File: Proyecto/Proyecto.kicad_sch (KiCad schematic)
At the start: 48 parts, among them IC1 MC9S08MP16xLC, J1 Bomba1, J10 DHT11, J11 Bomba2, J12 Aux1, J13 LCD, J14 Aux2, J15 Expansion, J16 NIVEL BAJO, J17 NIVEL ALTO, J18 LDR, J2 Rele1, J3 Luces, J4 Rele2, J5 TDS, J6 Rele3, J7 Rele4, J8 ENTRADA, J9 PH, K1 FINDER-36.11, K2 FINDER-36.11, K3 FINDER-36.11, K4 FINDER-36.11, Q1 IRF3205, Q2 IRF3205, U1 ULN2803A, U2 MIC4427, U3 AP63205WU, U4 PC817, U5 PC817, U6 LM358, U7 LM358

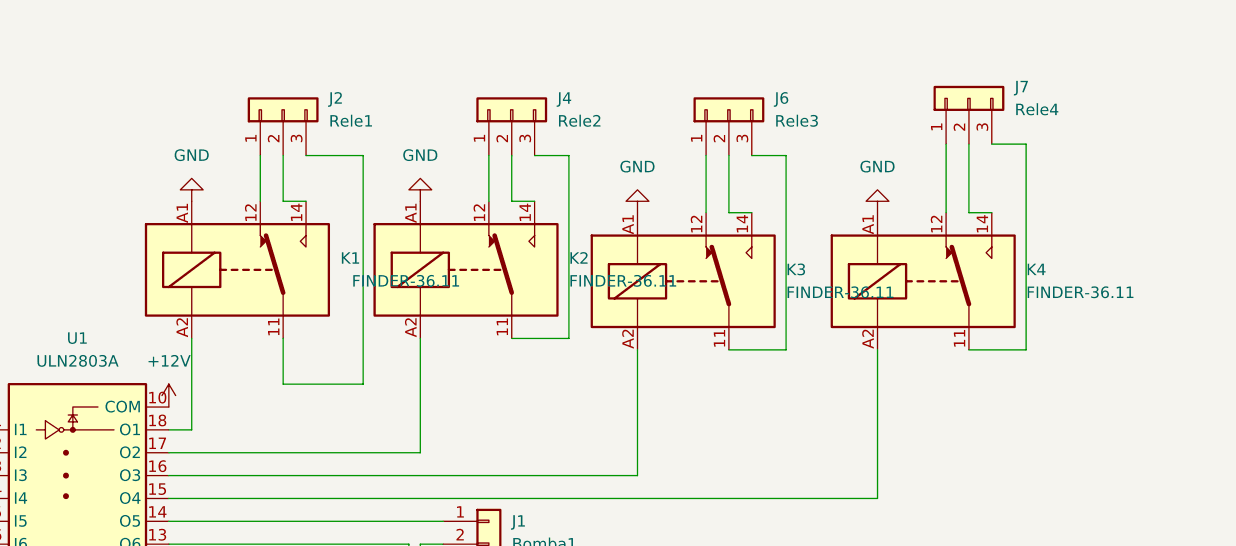
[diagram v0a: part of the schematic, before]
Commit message: 7-8-2022 itLA
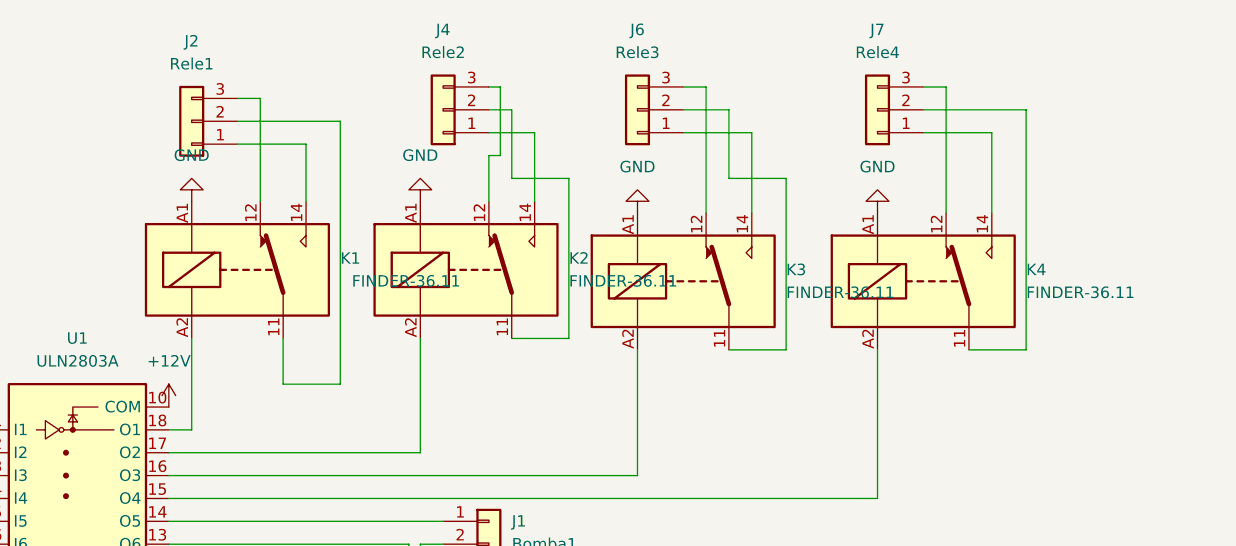
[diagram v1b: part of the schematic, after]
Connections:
- net at J7.1 (Pin_1): now also K4.14; no longer K4.12
- net at J7.2 (Pin_2): now also K4.11; no longer K4.14
- net at J7.3 (Pin_3): now also K4.12; no longer K4.11
- net at J4.1 (Pin_1): now also K2.14; no longer K2.12
- net at J4.2 (Pin_2): now also K2.11; no longer K2.14
- net at J4.3 (Pin_3): now also K2.12; no longer K2.11
- net at K3.11: now also J6.2 (Pin_2); no longer J6.3 (Pin_3)
- net at K3.12: now also J6.3 (Pin_3); no longer J6.1 (Pin_1)
- net at K3.14: now also J6.1 (Pin_1); no longer J6.2 (Pin_2)
- net at J2.1 (Pin_1): now also K1.14; no longer K1.12
- net at J2.2 (Pin_2): now also K1.11; no longer K1.14
- net at J2.3 (Pin_3): now also K1.12; no longer K1.11
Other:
- moved on the sheet: J2, J4, J6, J7

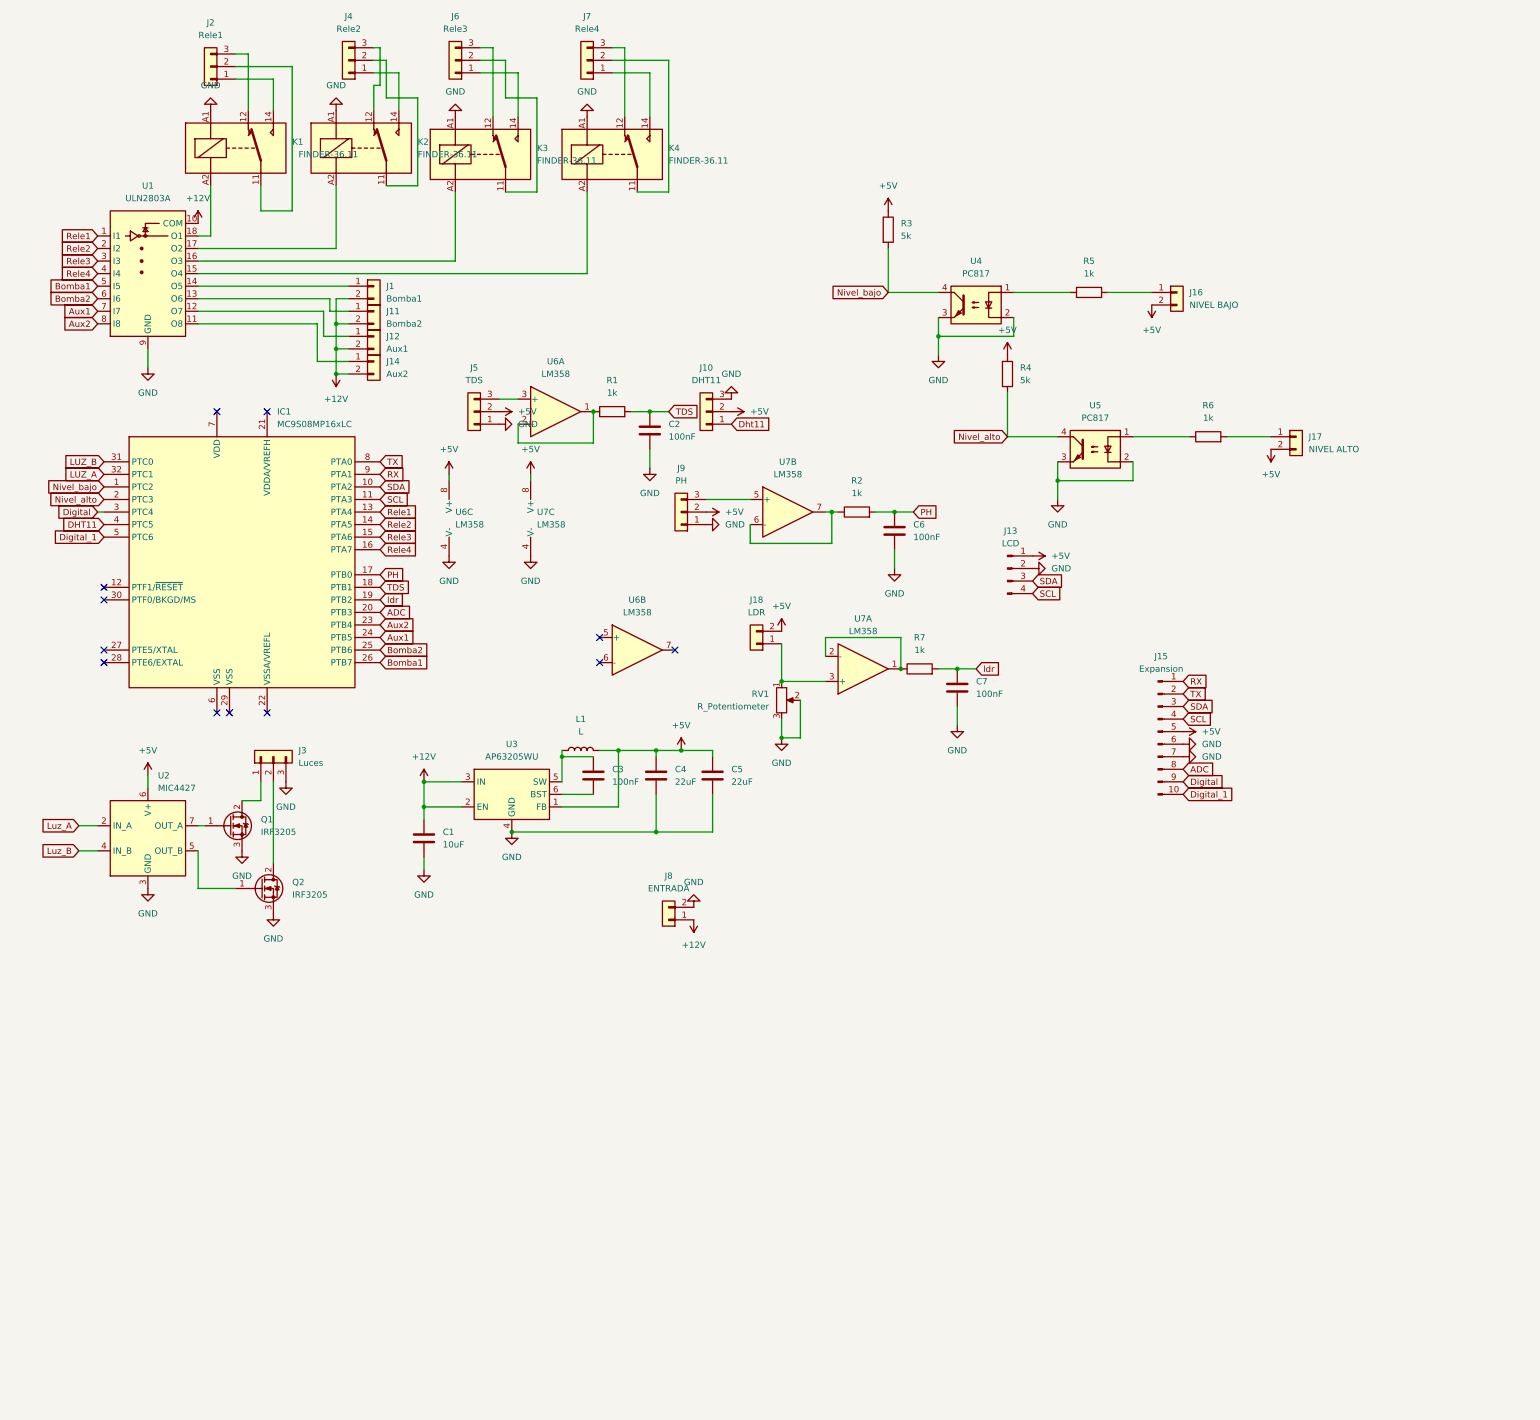
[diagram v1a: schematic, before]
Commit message: 15-7-2022
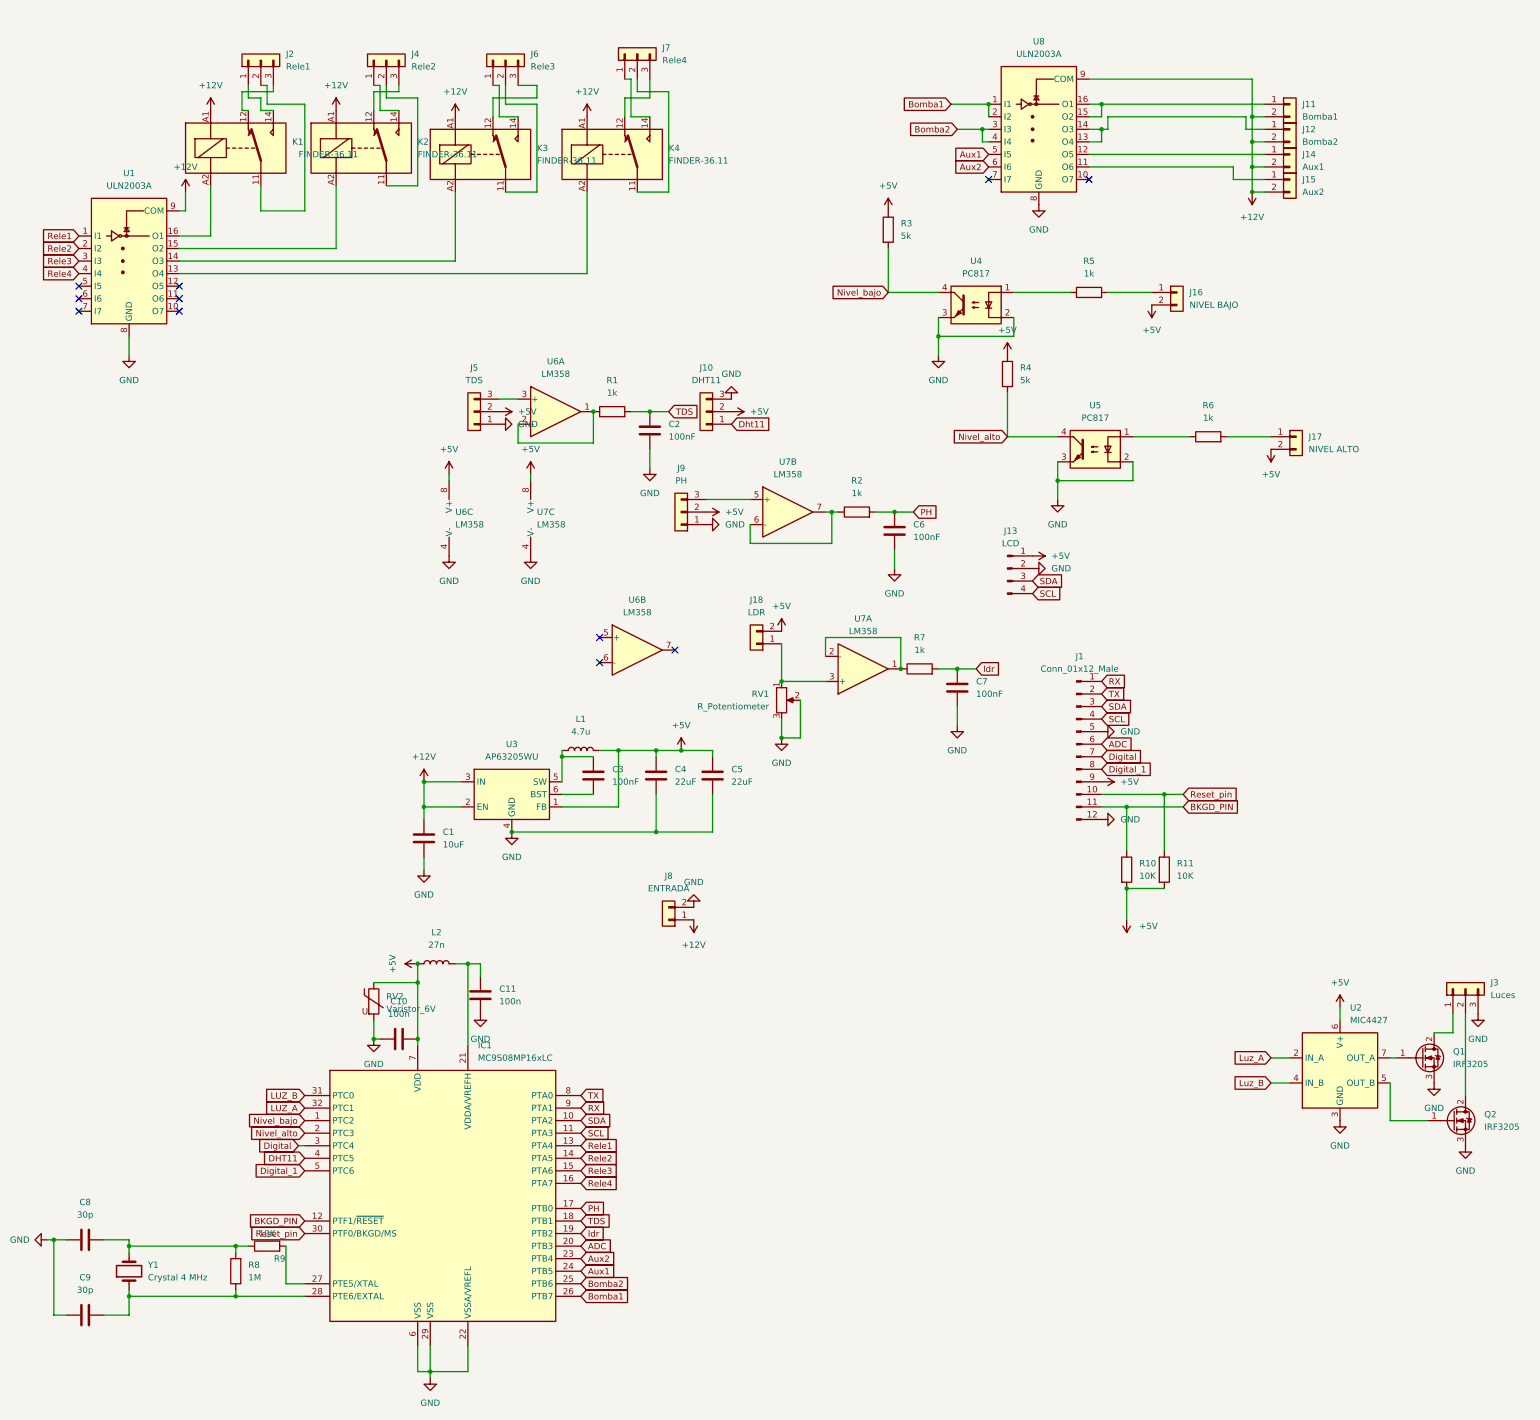
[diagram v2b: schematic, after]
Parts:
- removed J1: Bomba1, TerminalBlock:TerminalBlock_bornier-2_P5.08mm, symbol Connector_Generic:Conn_01x02
- removed J15: Expansion, Connector_PinHeader_1.00mm:PinHeader_1x10_P1.00mm_Vertical, symbol Connector:Conn_01x10_Male
- removed U1: ULN2803A, Package_SO:SOIC-18W_7.5x11.6mm_P1.27mm, symbol Transistor_Array:ULN2803A
- added C10, C11: 100n, Capacitor_SMD:C_0201_0603Metric, symbol Device:C
- added C8, C9: 30p, Capacitor_SMD:C_0201_0603Metric, symbol Device:C
- added J1: Conn_01x12_Male, Connector_PinHeader_2.54mm:PinHeader_1x12_P2.54mm_Vertical, symbol Connector:Conn_01x12_Male
- added J15: Aux2, TerminalBlock:TerminalBlock_bornier-2_P5.08mm, symbol Connector_Generic:Conn_01x02
- added L2: 27n, Inductor_SMD:L_0805_2012Metric, symbol Device:L
- added R10, R11, R9: 10K, Resistor_SMD:R_0201_0603Metric, symbol Device:R
- added R8: 1M, Resistor_SMD:R_0201_0603Metric, symbol Device:R
- added RV2: Varistor_6V, Capacitor_SMD:C_0805_2012Metric, symbol Device:Varistor
- added U1, U8: ULN2003A, Package_SO:SOIC-16_3.9x9.9mm_P1.27mm, symbol Transistor_Array:ULN2003A
- added Y1: Crystal 4 MHz, Crystal:Crystal_HC49-4H_Vertical, symbol Device:Crystal
- C1, C4, C5: footprint Capacitor_SMD:C_0603_1608Metric -> Capacitor_SMD:C_0805_2012Metric
- C3: footprint Capacitor_SMD:C_0603_1608Metric -> Capacitor_SMD:C_0201_0603Metric
- J11: value Bomba2 -> Bomba1
- J12: value Aux1 -> Bomba2
- J14: value Aux2 -> Aux1
- L1: value L -> 4.7u; footprint Inductor_SMD:L_0603_1608Metric -> Inductor_SMD:L_Bourns_SRN6045TA
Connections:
- net +12V: now also K1.A1, K2.A1, K3.A1, K4.A1, J15.2 (Pin_2), U1.9 (COM), U8.9 (COM)
- net +5V: now also IC1.7 (VDD), C10.2, J1.9 (Pin_9), L2.1, R10.2, R11.2, RV2.1
- net ADC: now also J1.6 (Pin_6)
- net Aux1: now also U8.5 (I5)
- net Aux2: now also U8.6 (I6)
- net Bomba1: now also U8.1 (I1), U8.2 (I2)
- net Bomba2: now also U8.3 (I3), U8.4 (I4)
- net Digital: now also J1.7 (Pin_7)
- net Digital_1: now also J1.8 (Pin_8)
- net GND: now also IC1.22 (VSSA/VREFL), IC1.29 (VSS), IC1.6 (VSS), C10.1, C11.1, C8.1, C9.1, J1.12 (Pin_12), J1.5 (Pin_5), RV2.2, U1.8 (GND), U8.8 (GND); no longer K1.A1, K2.A1, K3.A1, K4.A1
- net RX: now also J1.1 (Pin_1)
- net Rele1: now also U1.1 (I1)
- net Rele2: now also U1.2 (I2)
- net Rele3: now also U1.3 (I3)
- net Rele4: now also U1.4 (I4)
- net SCL: now also J1.4 (Pin_4)
- net SDA: now also J1.3 (Pin_3)
- net TX: now also J1.2 (Pin_2)
- net at J14.1 (Pin_1): now also U8.12 (O5)
- net BKGD_PIN: now reaches IC1.12 (PTF1/~{RESET})
- net BKGD_PIN: now also J1.11 (Pin_11), R10.1
- net at IC1.21 (VDDA/VREFH): now also C11.2, L2.2
- net at IC1.27 (PTE5/XTAL): now also R9.2
- net at IC1.28 (PTE6/EXTAL): now also C9.2, R8.1, Y1.1
- net Reset_pin: now reaches IC1.30 (PTF0/BKGD/MS)
- net Reset_pin: now also J1.10 (Pin_10), R11.1
- net at J12.1 (Pin_1): now also U8.13 (O4), U8.14 (O3)
- net at J11.1 (Pin_1): now also U8.15 (O2), U8.16 (O1)
- net at K4.A2: now also U1.13 (O4)
- net at K3.A2: now also U1.14 (O3)
- net at K2.A2: now also U1.15 (O2)
- net at K1.A2: now also U1.16 (O1)
- new net: C8.2, R8.2, R9.1, Y1.2
- new net: J15.1 (Pin_1), U8.11 (O6)
- no-connect marks 12 -> 11
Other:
- moved on the sheet: IC1, J2, J3, J4, J6, J7, Q1, Q2, U2
